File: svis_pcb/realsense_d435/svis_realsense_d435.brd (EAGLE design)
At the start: 10 parts

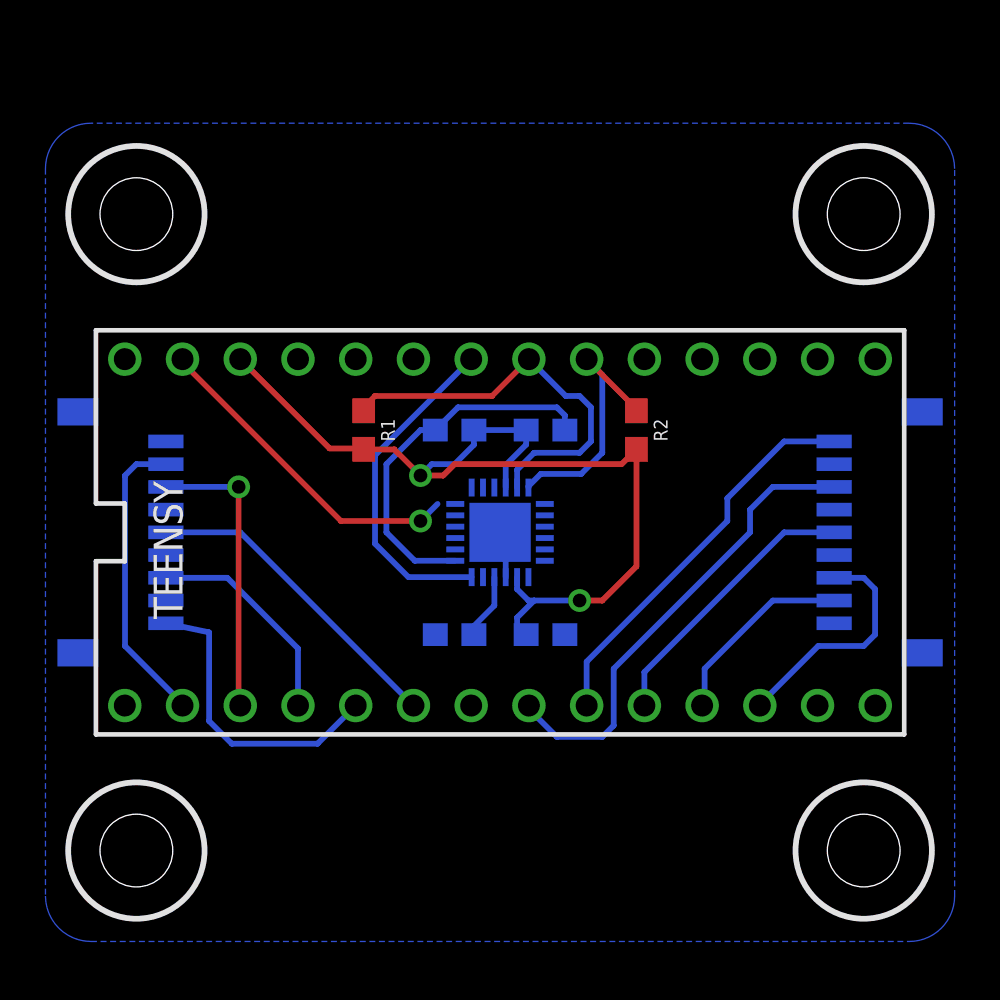
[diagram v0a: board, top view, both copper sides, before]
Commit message: Incorporate Samir's comments
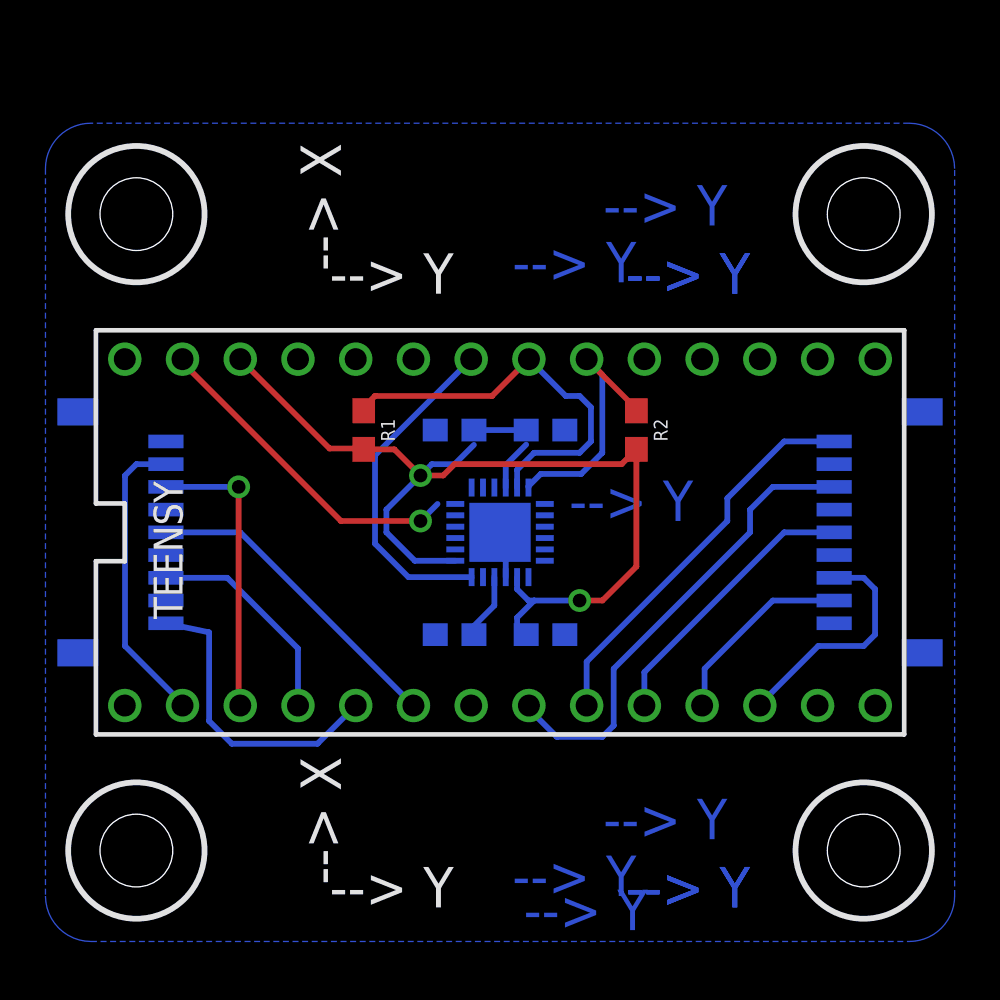
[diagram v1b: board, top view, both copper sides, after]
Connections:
- removed net N$2: C2.2, C3.2, ICM20689.13
- net 3.3V: now also ICM20689.13
- net GND: now also C2.2, C3.2
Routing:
- net N$2: track 16.2 -> 0.00 mm
- net 3.3V: track 42.7 -> 48.1 mm
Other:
- board text added: "--> X"
- board text added: "--> Y"
- board text added: "Y <--"
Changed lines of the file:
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@@
 <hole x="36" y="4" drill="3.2"/>
 <circle x="36" y="4" radius="3" width="0.254" layer="21"/>
+<text x="31" y="1.5" size="1.778" layer="16" rot="MR0">Y &lt;--</text>
+<text x="31" y="1.5" size="1.778" layer="16" rot="MR0">Y &lt;--</text>
+<text x="28.5" y="18.5" size="1.778" layer="16" rot="MR0">Y &lt;--</text>
+<text x="30" y="4.5" size="1.778" layer="16" rot="MR0">Y &lt;--</text>
+<text x="26" y="2" size="1.778" layer="16" rot="MR0">Y &lt;--</text>
+<text x="26.5" y="0.5" size="1.778" layer="16" rot="MR0">Y &lt;--</text>
+<text x="31.5" y="1.5" size="1.778" layer="26" rot="MR0">Y &lt;--</text>
+<text x="25" y="2.5" size="1.778" layer="26" rot="MR90">--&gt; X</text>
+<text x="31" y="28.5" size="1.778" layer="16" rot="MR0">Y &lt;--</text>
+<text x="31" y="28.5" size="1.778" layer="16" rot="MR0">Y &lt;--</text>
+<text x="30" y="31.5" size="1.778" layer="16" rot="MR0">Y &lt;--</text>
+<text x="26" y="29" size="1.778" layer="16" rot="MR0">Y &lt;--</text>
+<text x="31.5" y="28.5" size="1.778" layer="26" rot="MR0">Y &lt;--</text>
+<text x="25" y="29.5" size="1.778" layer="26" rot="MR90">--&gt; X</text>
+<text x="12.5" y="28.5" size="1.778" layer="25">--&gt; Y</text>
+<text x="12.5" y="1.5" size="1.778" layer="25">--&gt; Y</text>
+<text x="13" y="2.5" size="1.778" layer="25" rot="R90">--&gt; X</text>
+<text x="13" y="29.5" size="1.778" layer="25" rot="R90">--&gt; X</text>
 </plain>
 <attributes>
@@
 <wire x1="6.03" y1="25.47" x2="13" y2="18.5" width="0.254" layer="1"/>
 <wire x1="13" y1="18.5" x2="16.5" y2="18.5" width="0.254" layer="1"/>
+<contactref element="C2" pad="2"/>
+<contactref element="C3" pad="2"/>
 </signal>
 <signal name="3.3V">
@@
 <contactref element="R1" pad="2"/>
 <contactref element="R2" pad="2"/>
-<contactref element="C3" pad="1"/>
-<contactref element="C2" pad="1"/>
 <contactref element="ICM20689" pad="8"/>
 <contactref element="C4" pad="2"/>
 <contactref element="ICM20689" pad="22"/>
 <wire x1="12.5" y1="21.69" x2="8.57" y2="25.62" width="0.254" layer="1"/>
-<wire x1="21.15" y1="22.5" x2="21.15" y2="21.86" width="0.254" layer="16"/>
 <wire x1="21.15" y1="21.86" x2="20.25" y2="20.96" width="0.254" layer="16"/>
 <wire x1="20.25" y1="20.96" x2="20.25" y2="19.97" width="0.254" layer="16"/>
-<wire x1="18.85" y1="22.5" x2="21.15" y2="22.5" width="0.254" layer="16"/>
-<wire x1="18.85" y1="22.5" x2="18.85" y2="22.35" width="0.254" layer="16"/>
 <via x="16.5" y="20.5" extent="1-16" drill="0.6"/>
 <wire x1="26" y1="21.65" x2="26" y2="16.5" width="0.254" layer="1"/>
@@
 <wire x1="25.35" y1="21" x2="26" y2="21.65" width="0.254" layer="1"/>
 <wire x1="25.35" y1="21" x2="18" y2="21" width="0.254" layer="1"/>
-<wire x1="18.85" y1="21.85" x2="18.85" y2="22.5" width="0.254" layer="16"/>
 <wire x1="14" y1="21.65" x2="15.35" y2="21.65" width="0.254" layer="1"/>
 <wire x1="15.35" y1="21.65" x2="16.5" y2="20.5" width="0.254" layer="1"/>
@@
 <wire x1="17" y1="21" x2="18" y2="21" width="0.254" layer="16"/>
 <wire x1="18" y1="21" x2="18.85" y2="21.85" width="0.254" layer="16"/>
+<contactref element="C3" pad="1"/>
+<contactref element="C2" pad="1"/>
+<wire x1="18.85" y1="22.5" x2="21.15" y2="22.5" width="0.254" layer="16"/>
+<wire x1="18.85" y1="22.5" x2="18.85" y2="22.35" width="0.254" layer="16"/>
+<contactref element="ICM20689" pad="13"/>
+<wire x1="18.03" y1="16.75" x2="16.25" y2="16.75" width="0.254" layer="16"/>
+<wire x1="16.25" y1="16.75" x2="15" y2="18" width="0.254" layer="16"/>
+<wire x1="15" y1="19" x2="16.5" y2="20.5" width="0.254" layer="16"/>
+<wire x1="15" y1="19" x2="15" y2="18" width="0.254" layer="16"/>
+<wire x1="18.85" y1="21.85" x2="18.85" y2="22.35" width="0" layer="19" extent="16-16"/>
+<wire x1="21.15" y1="21.86" x2="21.15" y2="22.5" width="0" layer="19" extent="16-16"/>
 </signal>
 <signal name="VIN">
@@
 <wire x1="22.89" y1="24" x2="21.27" y2="25.62" width="0.254" layer="16"/>
 </signal>
-<signal name="N$2">
-<contactref element="ICM20689" pad="13"/>
-<contactref element="C3" pad="2"/>
-<contactref element="C2" pad="2"/>
-<wire x1="22.85" y1="22.5" x2="22.85" y2="23.15" width="0.254" layer="16"/>
-<wire x1="22.85" y1="23.15" x2="22.5" y2="23.5" width="0.254" layer="16"/>
-<wire x1="22.5" y1="23.5" x2="18.15" y2="23.5" width="0.254" layer="16"/>
-<wire x1="18.15" y1="23.5" x2="17.15" y2="22.5" width="0.254" layer="16"/>
-<wire x1="15" y1="18" x2="16.25" y2="16.75" width="0.254" layer="16"/>
-<wire x1="16.25" y1="16.75" x2="18.03" y2="16.75" width="0.254" layer="16"/>
-<wire x1="15" y1="21" x2="16.5" y2="22.5" width="0.254" layer="16"/>
-<wire x1="16.5" y1="22.5" x2="17.15" y2="22.5" width="0.254" layer="16"/>
-<wire x1="15" y1="18" x2="15" y2="21" width="0.254" layer="16"/>
-</signal>
 <signal name="N$1">
